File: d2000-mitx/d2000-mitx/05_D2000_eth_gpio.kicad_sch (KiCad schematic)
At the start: 3 parts, among them J8 RJ45_RB1-125B8G1A

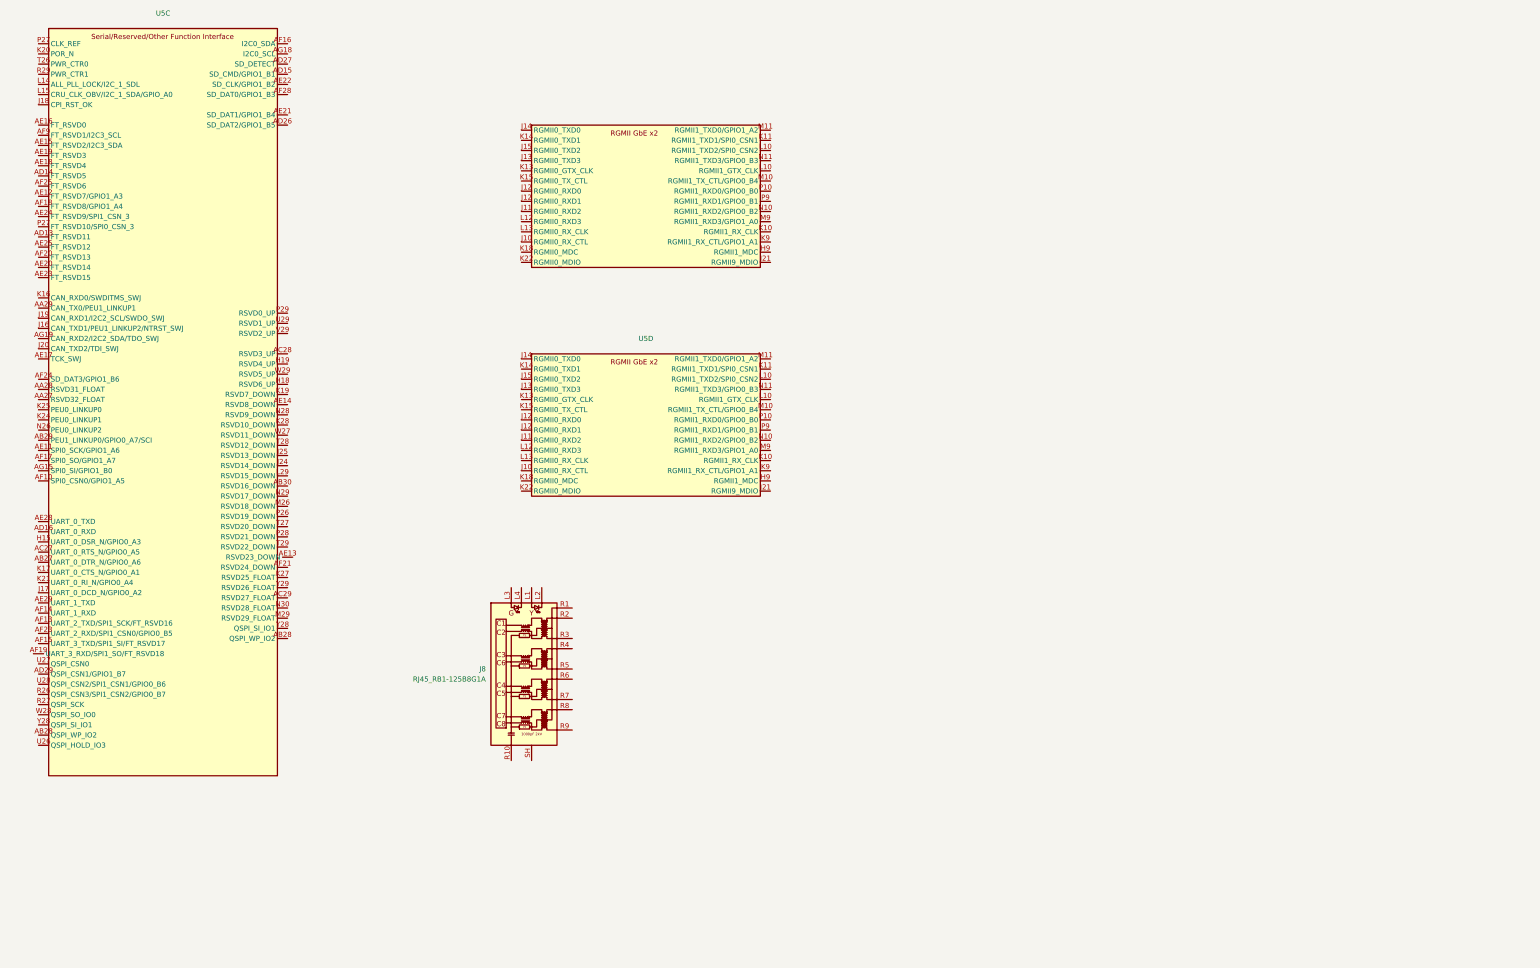
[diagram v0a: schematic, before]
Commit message: update schem + pcb layout
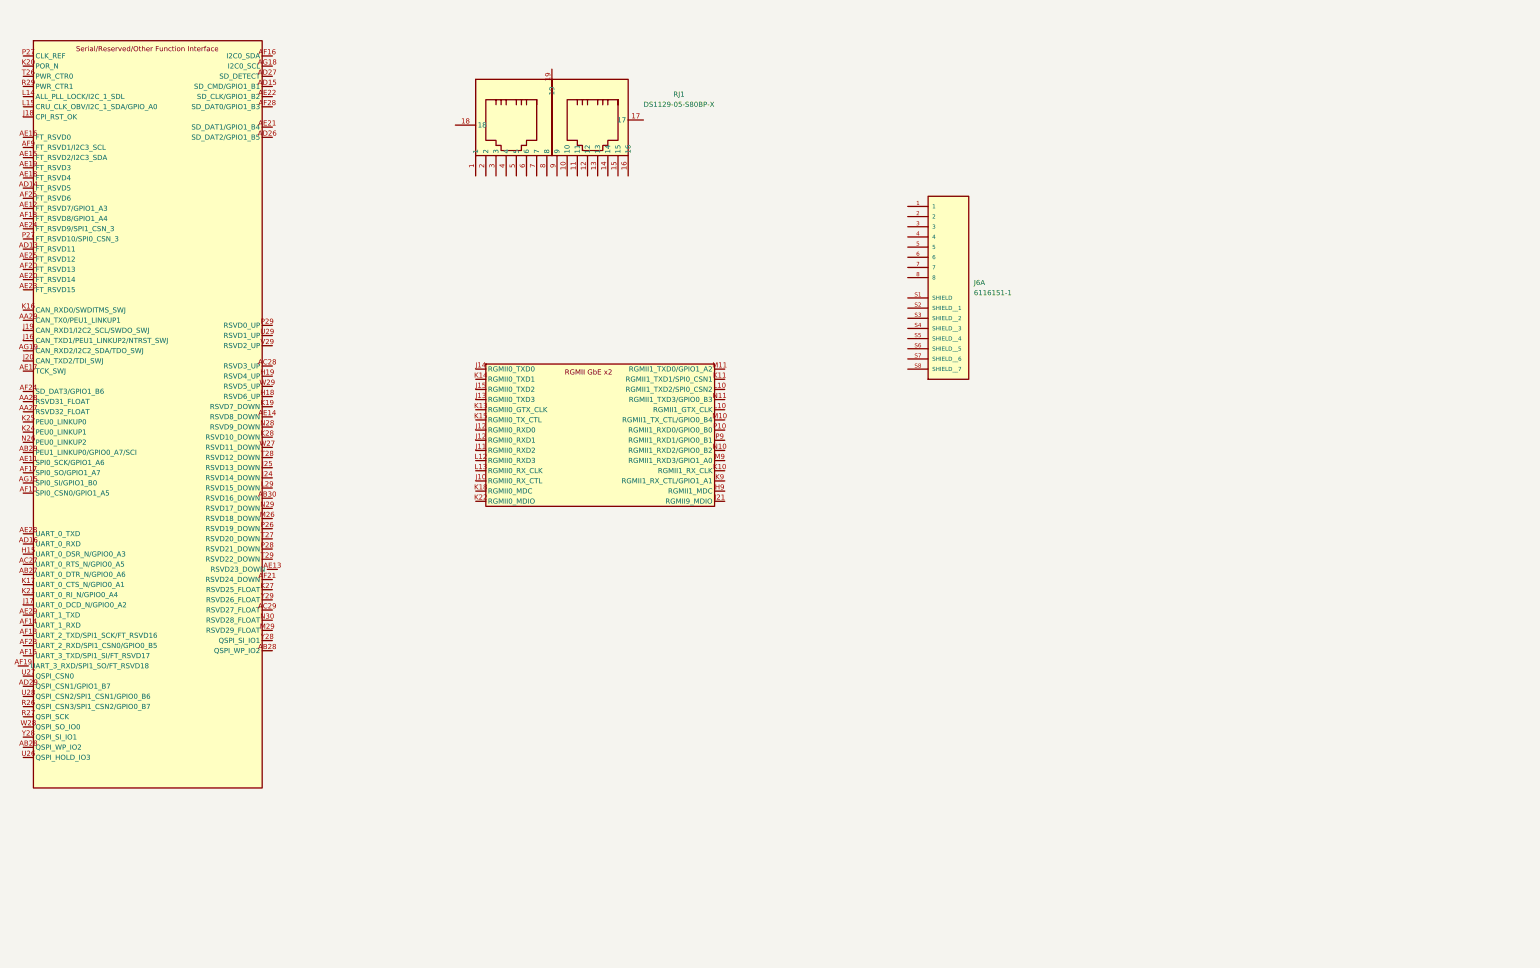
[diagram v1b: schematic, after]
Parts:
- removed J8: RJ45_RB1-125B8G1A, Connector_RJ:RJ45_UDE_RB1-125B8G1A, symbol Connector:RJ45_RB1-125B8G1A
- removed U3, U5: ~, symbol D2000:D2000-E8
- added J6: 6116151-1, 6116151_1:TE_6116151-1, symbol 6116151-1:6116151-1
- added RJ1: DS1129-05-S80BP-X, CONNFLY-Elec-DS1129-05-S80BP-X:RJ45-TH_DS1129-05-S80BP-X, symbol CONNFLY-Elec-DS1129-05-S80BP-X:DS1129-05-S80BP-X
- added U5: ~, D2000:D2000_DDR4_BGA1144P100_3500X350, symbol D2000-FT20004:D2000-E8

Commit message: update schem + pcb layout
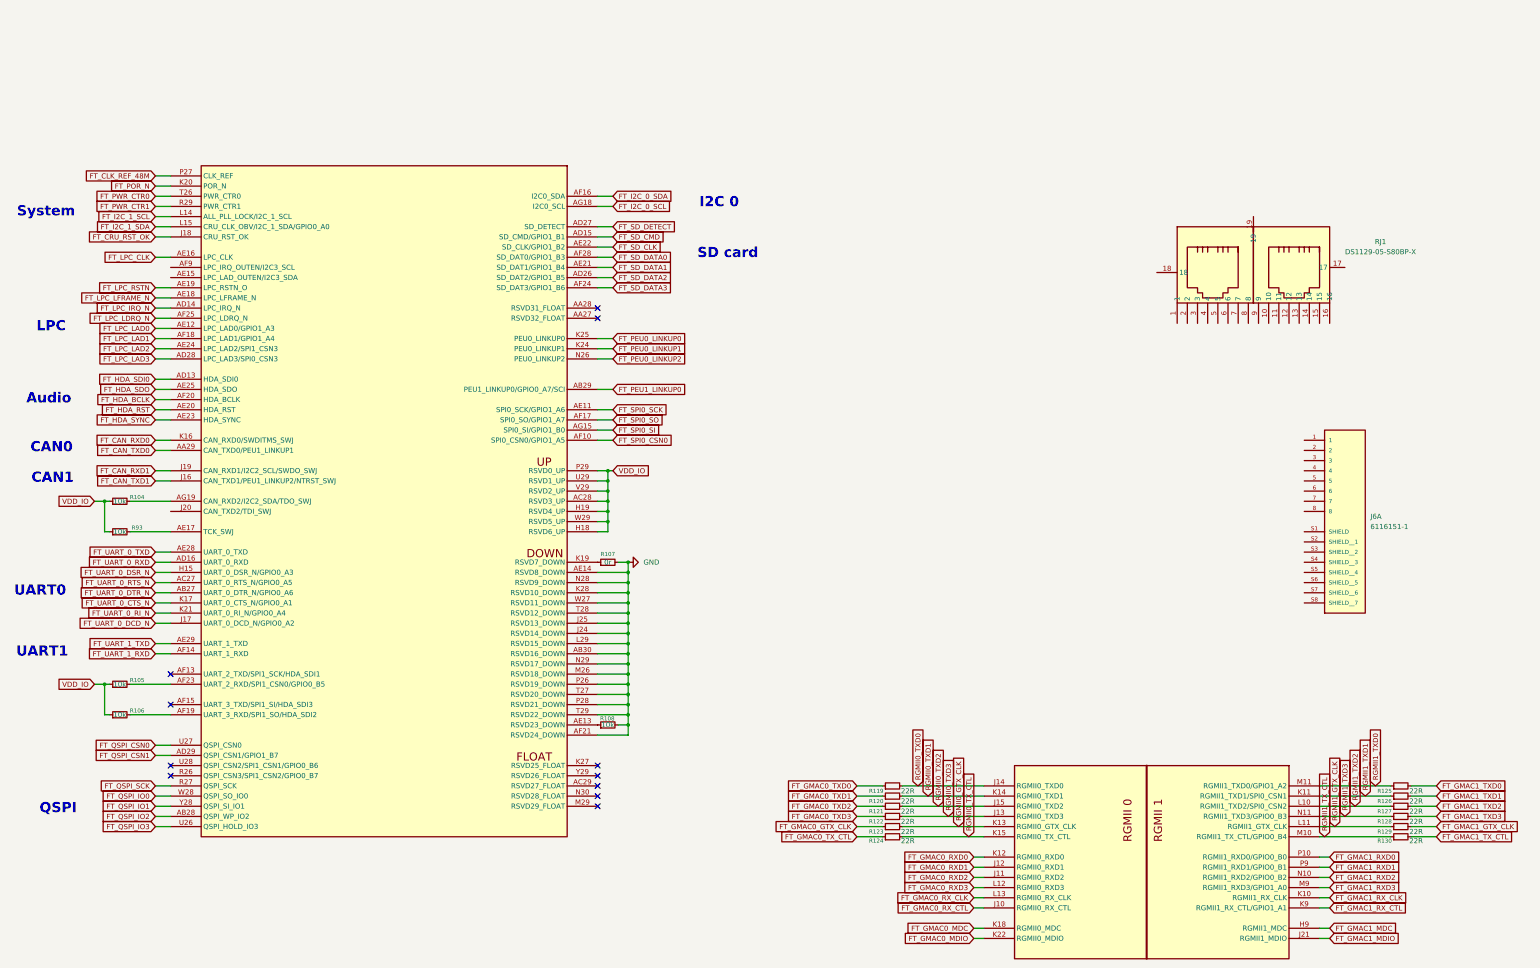
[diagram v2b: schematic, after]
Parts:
- added R104, R105, R106, R108, R93: 10k, Resistor_SMD:R_0402_1005Metric, symbol Device:R_Small
- added R107: 0r, Resistor_SMD:R_0402_1005Metric, symbol Device:R_Small
- added R119, R120, R121, R122, R123, R124, R125, R126, R127, R128, R129, R130: 22R, Resistor_SMD:R_0402_1005Metric, symbol Device:R_Small
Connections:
- net FT_GMAC1_MDC: now reaches U5.H9 (RGMII1_MDC)
- net FT_GMAC0_RX_CTL: now reaches U5.J10 (RGMII0_RX_CTL)
- net FT_GMAC0_RXD2: now reaches U5.J11 (RGMII0_RXD2)
- net FT_GMAC0_RXD1: now reaches U5.J12 (RGMII0_RXD1)
- net RGMII0_TXD3: now reaches U5.J13 (RGMII0_TXD3)
- net RGMII0_TXD3: now also R122.2
- net RGMII0_TXD0: now reaches U5.J14 (RGMII0_TXD0)
- net RGMII0_TXD0: now also R119.2
- net RGMII0_TXD2: now reaches U5.J15 (RGMII0_TXD2)
- net RGMII0_TXD2: now also R121.2
- net FT_GMAC1_MDIO: now reaches U5.J21 (RGMII1_MDIO)
- net FT_GMAC1_RX_CLK: now reaches U5.K10 (RGMII1_RX_CLK)
- net RGMII1_TXD1: now reaches U5.K11 (RGMII1_TXD1/SPI0_CSN1)
- net RGMII1_TXD1: now also R126.1
- net RGMII0_GTX_CLK: now reaches U5.K13 (RGMII0_GTX_CLK)
- net RGMII0_GTX_CLK: now also R123.2
- net RGMII0_TXD1: now reaches U5.K14 (RGMII0_TXD1)
- net RGMII0_TXD1: now also R120.2
- net RGMII0_TX_CTL: now reaches U5.K15 (RGMII0_TX_CTL)
- net RGMII0_TX_CTL: now also R124.2
- net FT_GMAC0_MDC: now reaches U5.K18 (RGMII0_MDC)
- net FT_GMAC0_MDIO: now reaches U5.K22 (RGMII0_MDIO)
- net FT_GMAC1_RX_CTL: now reaches U5.K9 (RGMII1_RX_CTL/GPIO1_A1)
- net RGMII1_TXD2: now reaches U5.L10 (RGMII1_TXD2/SPI0_CSN2)
- net RGMII1_TXD2: now also R127.1
- net FT_GMAC0_RXD3: now reaches U5.L12 (RGMII0_RXD3)
- net FT_GMAC0_RX_CLK: now reaches U5.L13 (RGMII0_RX_CLK)
- net RGMII1_TX_CTL: now reaches U5.M10 (RGMII1_TX_CTL/GPIO0_B4)
- net RGMII1_TX_CTL: now also R130.1
- net RGMII1_TXD0: now reaches U5.M11 (RGMII1_TXD0/GPIO1_A2)
- net RGMII1_TXD0: now also R125.1
- net FT_GMAC1_RXD3: now reaches U5.M9 (RGMII1_RXD3/GPIO1_A0)
- net FT_GMAC1_RXD2: now reaches U5.N10 (RGMII1_RXD2/GPIO0_B2)
- net RGMII1_TXD3: now reaches U5.N11 (RGMII1_TXD3/GPIO0_B3)
- net RGMII1_TXD3: now also R128.1
- net FT_GMAC1_RXD0: now reaches U5.P10 (RGMII1_RXD0/GPIO0_B0)
- net FT_GMAC1_RXD1: now reaches U5.P9 (RGMII1_RXD1/GPIO0_B1)
- net FT_CAN_TXD0: now reaches U5.AA29 (CAN_TXD0/PEU1_LINKUP1)
- net FT_UART_0_DTR_N: now reaches U5.AB27 (UART_0_DTR_N/GPIO0_A6)
- net FT_QSPI_IO2: now reaches U5.AB28 (QSPI_WP_IO2)
- net FT_PEU1_LINKUP0: now reaches U5.AB29 (PEU1_LINKUP0/GPIO0_A7/SCI)
- net GND: now reaches U5.AB30 (RSVD16_DOWN)
- net GND: now also U5.AE14 (RSVD8_DOWN), U5.AF21 (RSVD24_DOWN), U5.J24 (RSVD14_DOWN), U5.J25 (RSVD13_DOWN), U5.K28 (RSVD10_DOWN), U5.L29 (RSVD15_DOWN), U5.M26 (RSVD18_DOWN), U5.N28 (RSVD9_DOWN), U5.N29 (RSVD17_DOWN), U5.P26 (RSVD19_DOWN), U5.P28 (RSVD21_DOWN), U5.T27 (RSVD20_DOWN), U5.T28 (RSVD12_DOWN), U5.T29 (RSVD22_DOWN), U5.W27 (RSVD11_DOWN), R107.2, R108.2
- net FT_UART_0_RTS_N: now reaches U5.AC27 (UART_0_RTS_N/GPIO0_A5)
- net VDD_IO: now reaches U5.AC28 (RSVD3_UP)
- net VDD_IO: now also U5.H18 (RSVD6_UP), U5.H19 (RSVD4_UP), U5.P29 (RSVD0_UP), U5.U29 (RSVD1_UP), U5.V29 (RSVD2_UP), U5.W29 (RSVD5_UP), R104.1, R105.1, R106.1, R93.1
- net FT_HDA_SDI0: now reaches U5.AD13 (HDA_SDI0)
- net FT_LPC_IRQ_N: now reaches U5.AD14 (LPC_IRQ_N)
- net FT_SD_CMD: now reaches U5.AD15 (SD_CMD/GPIO1_B1)
- net FT_UART_0_RXD: now reaches U5.AD16 (UART_0_RXD)
- net FT_SD_DATA2: now reaches U5.AD26 (SD_DAT2/GPIO1_B5)
- net FT_SD_DETECT: now reaches U5.AD27 (SD_DETECT)
- net FT_QSPI_CSN1: now reaches U5.AD29 (QSPI_CSN1/GPIO1_B7)
- net FT_SPI0_SCK: now reaches U5.AE11 (SPI0_SCK/GPIO1_A6)
- net FT_LPC_LAD0: now reaches U5.AE12 (LPC_LAD0/GPIO1_A3)
- net at U5.AE13 (RSVD23_DOWN): now also R108.1
- net FT_LPC_CLK: now reaches U5.AE16 (LPC_CLK)
- net at U5.AE17 (TCK_SWJ): now also R93.2
- net FT_LPC_LFRAME_N: now reaches U5.AE18 (LPC_LFRAME_N)
- net FT_LPC_RSTN: now reaches U5.AE19 (LPC_RSTN_O)
- net FT_HDA_RST: now reaches U5.AE20 (HDA_RST)
- net FT_SD_DATA1: now reaches U5.AE21 (SD_DAT1/GPIO1_B4)
- net FT_SD_CLK: now reaches U5.AE22 (SD_CLK/GPIO1_B2)
- net FT_HDA_SYNC: now reaches U5.AE23 (HDA_SYNC)
- net FT_LPC_LAD2: now reaches U5.AE24 (LPC_LAD2/SPI1_CSN3)
- net FT_HDA_SDO: now reaches U5.AE25 (HDA_SDO)
- net FT_UART_0_TXD: now reaches U5.AE28 (UART_0_TXD)
- net FT_UART_1_TXD: now reaches U5.AE29 (UART_1_TXD)
- net FT_SPI0_CSN0: now reaches U5.AF10 (SPI0_CSN0/GPIO1_A5)
- net FT_UART_1_RXD: now reaches U5.AF14 (UART_1_RXD)
- net FT_I2C_0_SDA: now reaches U5.AF16 (I2C0_SDA)
- net FT_SPI0_SO: now reaches U5.AF17 (SPI0_SO/GPIO1_A7)
- net FT_LPC_LAD1: now reaches U5.AF18 (LPC_LAD1/GPIO1_A4)
- net at U5.AF19 (UART_3_RXD/SPI1_SO/HDA_SDI2): now also R106.2
- net FT_HDA_BCLK: now reaches U5.AF20 (HDA_BCLK)
- net at U5.AF23 (UART_2_RXD/SPI1_CSN0/GPIO0_B5): now also R105.2
- net FT_SD_DATA3: now reaches U5.AF24 (SD_DAT3/GPIO1_B6)
- net FT_LPC_LDRQ_N: now reaches U5.AF25 (LPC_LDRQ_N)
- net FT_SD_DATA0: now reaches U5.AF28 (SD_DAT0/GPIO1_B3)
- net FT_SPI0_SI: now reaches U5.AG15 (SPI0_SI/GPIO1_B0)
- net FT_I2C_0_SCL: now reaches U5.AG18 (I2C0_SCL)
- net at U5.AG19 (CAN_RXD2/I2C2_SDA/TDO_SWJ): now also R104.2
- net FT_UART_0_DSR_N: now reaches U5.H15 (UART_0_DSR_N/GPIO0_A3)
- net FT_CAN_TXD1: now reaches U5.J16 (CAN_TXD1/PEU1_LINKUP2/NTRST_SWJ)
- net FT_UART_0_DCD_N: now reaches U5.J17 (UART_0_DCD_N/GPIO0_A2)
- net FT_CRU_RST_OK: now reaches U5.J18 (CRU_RST_OK)
- net FT_CAN_RXD1: now reaches U5.J19 (CAN_RXD1/I2C2_SCL/SWDO_SWJ)
- net FT_CAN_RXD0: now reaches U5.K16 (CAN_RXD0/SWDITMS_SWJ)
- net FT_UART_0_CTS_N: now reaches U5.K17 (UART_0_CTS_N/GPIO0_A1)
- net at U5.K19 (RSVD7_DOWN): now also R107.1
- net FT_POR_N: now reaches U5.K20 (POR_N)
- net FT_UART_0_RI_N: now reaches U5.K21 (UART_0_RI_N/GPIO0_A4)
- net FT_PEU0_LINKUP1: now reaches U5.K24 (PEU0_LINKUP1)
- net FT_PEU0_LINKUP0: now reaches U5.K25 (PEU0_LINKUP0)
- net FT_I2C_1_SCL: now reaches U5.L14 (ALL_PLL_LOCK/I2C_1_SCL)
- net FT_I2C_1_SDA: now reaches U5.L15 (CRU_CLK_OBV/I2C_1_SDA/GPIO0_A0)
- net FT_PEU0_LINKUP2: now reaches U5.N26 (PEU0_LINKUP2)
- net FT_CLK_REF_48M: now reaches U5.P27 (CLK_REF)
- net FT_QSPI_SCK: now reaches U5.R27 (QSPI_SCK)
- net FT_PWR_CTR1: now reaches U5.R29 (PWR_CTR1)
- net FT_PWR_CTR0: now reaches U5.T26 (PWR_CTR0)
- net FT_QSPI_IO3: now reaches U5.U26 (QSPI_HOLD_IO3)
- net FT_QSPI_CSN0: now reaches U5.U27 (QSPI_CSN0)
- net FT_QSPI_IO0: now reaches U5.W28 (QSPI_SO_IO0)
- net FT_QSPI_IO1: now reaches U5.Y28 (QSPI_SI_IO1)
- new net FT_GMAC0_GTX_CLK: R123.1
- new net FT_GMAC0_RXD0: U5.K12 (RGMII0_RXD0)
- new net FT_GMAC0_TXD0: R119.1
- new net FT_GMAC0_TXD1: R120.1
- new net FT_GMAC0_TXD2: R121.1
- new net FT_GMAC0_TXD3: R122.1
- new net FT_GMAC0_TX_CTL: R124.1
- new net FT_GMAC1_GTX_CLK: R129.2
- new net FT_GMAC1_TXD0: R125.2
- new net FT_GMAC1_TXD1: R126.2
- new net FT_GMAC1_TXD2: R127.2
- new net FT_GMAC1_TXD3: R128.2
- new net FT_GMAC1_TX_CTL: R130.2
- new net FT_LPC_LAD3: U5.AD28 (LPC_LAD3/SPI0_CSN3)
- new net RGMII1_GTX_CLK: R129.1, U5.L11 (RGMII1_GTX_CLK)
- no-connect marks 0 -> 11
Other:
- note added: "Audio"
- note added: "CAN0"
- note added: "CAN1"
- note added: "I2C 0"
- note added: "LPC"
- note added: "QSPI"
- note added: "SD card"
- note added: "System"
- note added: "UART0"
- note added: "UART1"
- moved on the sheet: J6A, RJ1
